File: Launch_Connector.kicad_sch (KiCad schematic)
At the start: 26 parts, among them J1 ADC1, J2 ADC2, J3 PWM, J4 GPIO

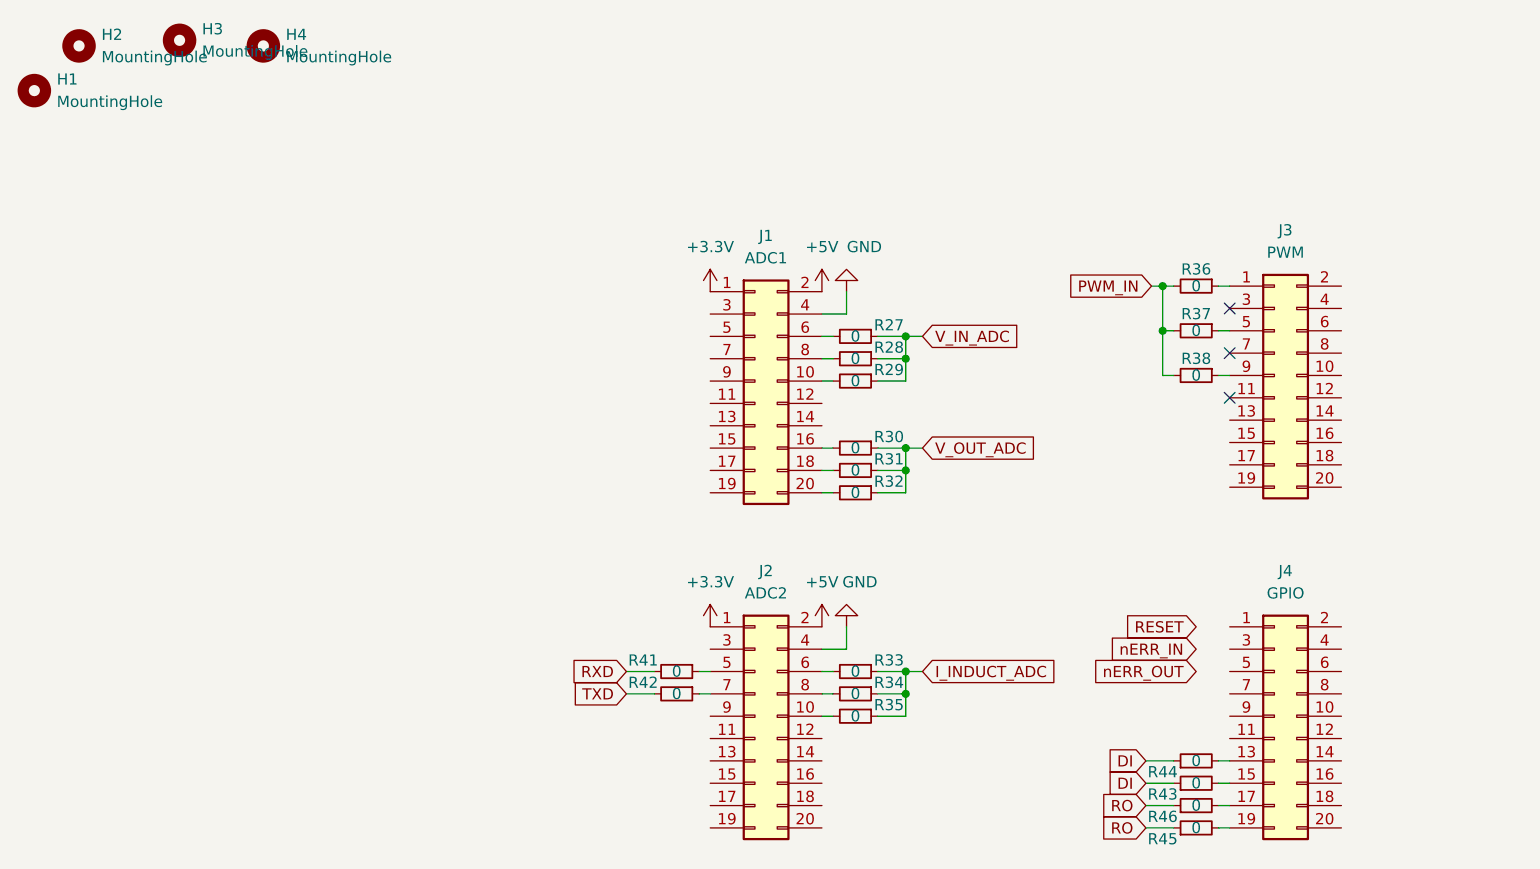
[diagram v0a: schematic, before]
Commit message: Первая версия в производство
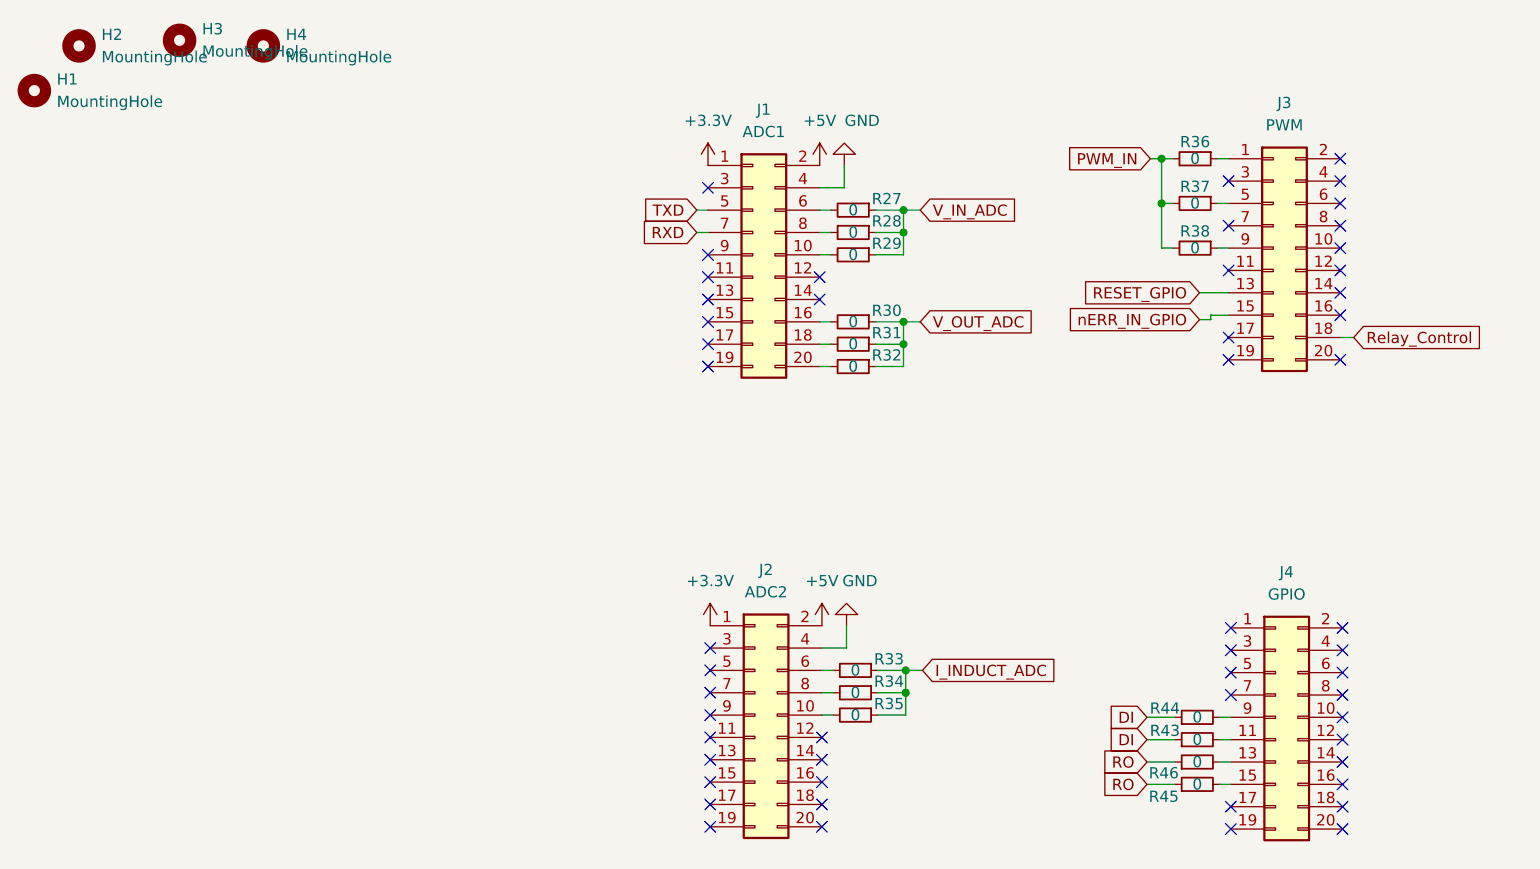
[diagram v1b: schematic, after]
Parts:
- removed R41, R42: 0, Resistor_SMD:R_0805_2012Metric_Pad1.20x1.40mm_HandSolder, symbol Device:R_Small
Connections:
- net RXD: now also J1.7 (Pin_7)
- net TXD: now also J1.5 (Pin_5)
- net at R45.2: now also J4.15 (Pin_15); no longer J4.19 (Pin_19)
- net at J4.11 (Pin_11): now also R43.2
- net at J4.13 (Pin_13): now also R46.2; no longer R44.2
- net at J4.17 (Pin_17): no longer R46.2
- net at J4.9 (Pin_9): now also R44.2
- net RESET_GPIO: now reaches J3.13 (Pin_13)
- net nERR_IN_GPIO: now reaches J3.15 (Pin_15)
- net Relay_Control: now reaches J3.18 (Pin_18)
- no-connect marks 3 -> 53
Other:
- moved on the sheet: J1, J3, R27, R28, R29, R30, R31, R32, R36, R37, R38, R43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
